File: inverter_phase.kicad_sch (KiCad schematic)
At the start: 34 parts, among them Q501 BSC072N08NS5, Q502 BSC072N08NS5, U501 IR2171S, U502 INA180B2

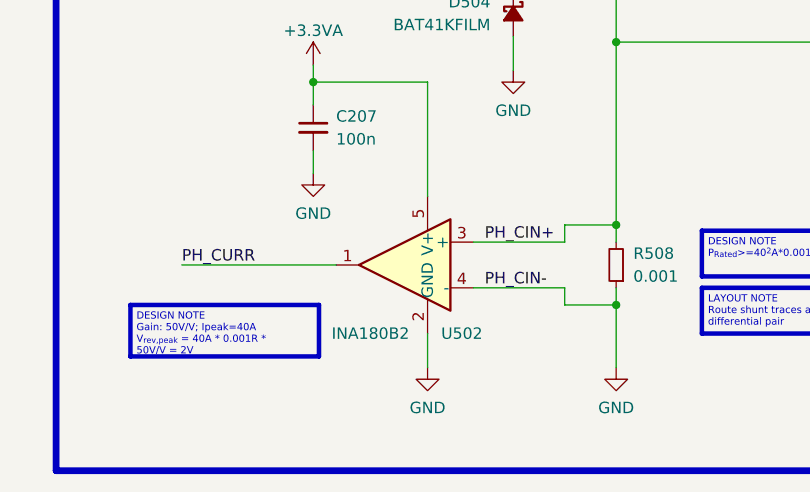
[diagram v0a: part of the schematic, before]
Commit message: feat: component placement, again
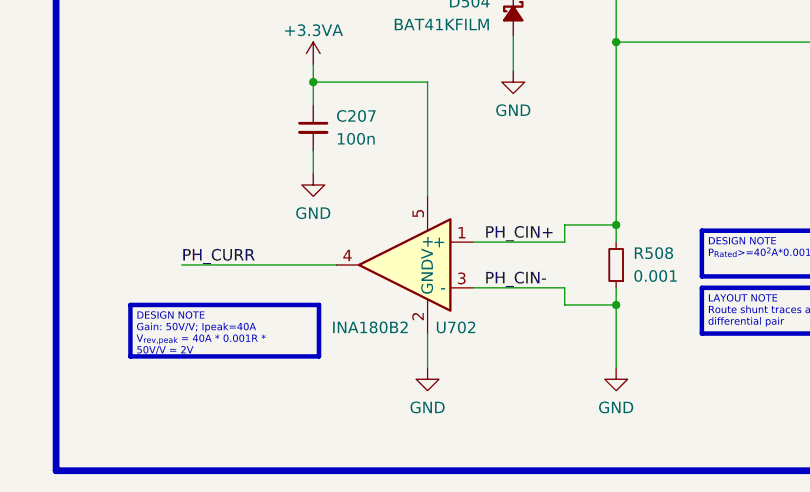
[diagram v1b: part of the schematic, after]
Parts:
- removed U502: INA180B2, Package_TO_SOT_SMD:SOT-23-5, symbol Amplifier_Current:INA180A2
- added U702: INA180B2, Package_TO_SOT_SMD:SOT-23-5, symbol Amplifier_Current:INA180B2
- C207: footprint Capacitor_SMD:C_0402_1005Metric_Pad0.74x0.62mm_HandSolder -> Capacitor_SMD:C_0805_2012Metric_Pad1.18x1.45mm_HandSolder
- C224: footprint Capacitor_SMD:C_0603_1608Metric_Pad1.08x0.95mm_HandSolder -> Capacitor_SMD:C_0805_2012Metric_Pad1.18x1.45mm_HandSolder
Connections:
- net +3.3VA: now also U702.5 (V+)
- net GND: now also U702.2 (GND), U702.3 (-)
- net PH_CIN+: now also U702.1 (+)
- net PH_CURR: now also U702.4
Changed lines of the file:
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@@
       (effects (font (size 1.27 1.27)) (justify left))
     )
-    (property "Footprint" "Capacitor_SMD:C_0402_1005Metric_Pad0.74x0.62mm_HandSolder" (at 257.175 86.995 0)
+    (property "Footprint" "Capacitor_SMD:C_0805_2012Metric_Pad1.18x1.45mm_HandSolder" (at 257.175 86.995 0)
       (effects (font (size 1.27 1.27)) hide)
     )
@@
       (effects (font (size 1.27 1.27)) (justify left))
     )
-    (property "Footprint" "Capacitor_SMD:C_0603_1608Metric_Pad1.08x0.95mm_HandSolder" (at 88.9 64.77 0)
+    (property "Footprint" "Capacitor_SMD:C_0805_2012Metric_Pad1.18x1.45mm_HandSolder" (at 88.9 64.77 0)
       (effects (font (size 1.27 1.27)) hide)
     )
@@
     )
   )
-  (symbol (lib_id "Device:C_Small") (at 102.235 64.77 180) (unit 1)
-    (in_bom yes) (on_board yes) (dnp no)
-    (property "Reference" "C502" (at 104.775 63.5 0)
-      (effects (font (size 1.27 1.27)) (justify right))
-    )
-    (property "Value" "100n 50V" (at 104.775 65.405 0)
-      (effects (font (size 1.27 1.27)) (justify right))
-    )
-    (property "Footprint" "Capacitor_SMD:C_0402_1005Metric_Pad0.74x0.62mm_HandSolder" (at 102.235 64.77 0)
-      (effects (font (size 1.27 1.27)) hide)
-    )
-    (property "Datasheet" "~" (at 102.235 64.77 0)
-      (effects (font (size 1.27 1.27)) hide)
-    )
-    (pin "1")
-    (pin "2")
-    (instances
-      (project "ESC_R1"
-        (path "/9dea2e18-5867-4ed4-a12d-7ee109225de0/a82201a8-9dca-4a1d-828e-2de3fb3c1adb"
-          (reference "C502") (unit 1)
-        )
-        (path "/9dea2e18-5867-4ed4-a12d-7ee109225de0/fe2fcbfe-ce2b-4fee-9243-f26c3dcbcd78"
-          (reference "C604") (unit 1)
-        )
-        (path "/9dea2e18-5867-4ed4-a12d-7ee109225de0/4eb0e494-3187-44db-9d3d-24d2fbf5dea7"
-          (reference "C704") (unit 1)
-        )
-      )
-    )
-  )
-  (symbol (lib_id "Device:C_Small") (at 107.95 139.065 180) (unit 1)
-    (in_bom yes) (on_board yes) (dnp no)
-    (property "Reference" "C509" (at 110.49 138.43 0)
-      (effects (font (size 1.27 1.27)) (justify right))
-    )
-    (property "Value" "10n" (at 110.49 140.335 0)
-      (effects (font (size 1.27 1.27)) (justify right))
-    )
-    (property "Footprint" "Capacitor_SMD:C_0603_1608Metric_Pad1.08x0.95mm_HandSolder" (at 107.95 139.065 0)
-      (effects (font (size 1.27 1.27)) hide)
-    )
-    (property "Datasheet" "~" (at 107.95 139.065 0)
-      (effects (font (size 1.27 1.27)) hide)
-    )
-    (pin "1")
-    (pin "2")
-    (instances
-      (project "ESC_R1"
-        (path "/9dea2e18-5867-4ed4-a12d-7ee109225de0/a82201a8-9dca-4a1d-828e-2de3fb3c1adb"
-          (reference "C509") (unit 1)
-        )
-        (path "/9dea2e18-5867-4ed4-a12d-7ee109225de0/fe2fcbfe-ce2b-4fee-9243-f26c3dcbcd78"
-          (reference "C609") (unit 1)
-        )
-        (path "/9dea2e18-5867-4ed4-a12d-7ee109225de0/4eb0e494-3187-44db-9d3d-24d2fbf5dea7"
-          (reference "C709") (unit 1)
-        )
-      )
-    )
-  )
-  (symbol (lib_id "Amplifier_Current:INA180A2") (at 207.645 138.43 0) (mirror y) (unit 1)
-    (in_bom yes) (on_board yes) (dnp no)
-    (property "Reference" "U502" (at 213.995 146.05 0)
-      (effects (font (size 1.27 1.27)))
-    )
-    (property "Value" "INA180B2" (at 203.835 146.05 0)
-      (effects (font (size 1.27 1.27)))
-    )
-    (property "Footprint" "Package_TO_SOT_SMD:SOT-23-5" (at 206.375 137.16 0)
-      (effects (font (size 1.27 1.27)) hide)
-    )
-    (property "Datasheet" "http://www.ti.com/lit/ds/symlink/ina180.pdf" (at 203.835 134.62 0)
-      (effects (font (size 1.27 1.27)) hide)
-    )
-    (property "Link" "https://www.digikey.de/en/products/detail/texas-instruments/INA180B2IDBVR/8105877" (at 207.645 138.43 0)
+  (symbol (lib_id "Amplifier_Current:INA180B2") (at 210.185 138.43 0) (mirror y) (unit 1)
+    (in_bom yes) (on_board yes) (dnp no)
+    (property "Reference" "U702" (at 213.36 145.415 0)
+      (effects (font (size 1.27 1.27)))
+    )
+    (property "Value" "INA180B2" (at 203.835 145.415 0)
+      (effects (font (size 1.27 1.27)))
+    )
+    (property "Footprint" "Package_TO_SOT_SMD:SOT-23-5" (at 210.185 138.43 0)
+      (effects (font (size 1.27 1.27)) hide)
+    )
+    (property "Datasheet" "" (at 210.185 138.43 0)
+      (effects (font (size 1.27 1.27)) hide)
+    )
+    (property "Link" "https://www.digikey.de/en/products/detail/texas-instruments/INA180B2IDBVR/8105877" (at 210.185 138.43 0)
       (effects (font (size 1.27 1.27)) hide)
     )
@@
     (instances
       (project "ESC_R1"
+        (path "/9dea2e18-5867-4ed4-a12d-7ee109225de0/4eb0e494-3187-44db-9d3d-24d2fbf5dea7"
+          (reference "U702") (unit 1)
+        )
         (path "/9dea2e18-5867-4ed4-a12d-7ee109225de0/a82201a8-9dca-4a1d-828e-2de3fb3c1adb"
           (reference "U502") (unit 1)
@@
           (reference "U602") (unit 1)
         )
-        (path "/9dea2e18-5867-4ed4-a12d-7ee109225de0/4eb0e494-3187-44db-9d3d-24d2fbf5dea7"
-          (reference "U702") (unit 1)
-        )
-      )
+      )
+    )
+  )
+  (symbol (lib_id "Device:C_Small") (at 102.235 64.77 180) (unit 1)
+    (in_bom yes) (on_board yes) (dnp no)
+    (property "Reference" "C502" (at 104.775 63.5 0)
+      (effects (font (size 1.27 1.27)) (justify right))
+    )
+    (property "Value" "100n 50V" (at 104.775 65.405 0)
+      (effects (font (size 1.27 1.27)) (justify right))
+    )
+    (property "Footprint" "Capacitor_SMD:C_0402_1005Metric_Pad0.74x0.62mm_HandSolder" (at 102.235 64.77 0)
+      (effects (font (size 1.27 1.27)) hide)
+    )
+    (property "Datasheet" "~" (at 102.235 64.77 0)
+      (effects (font (size 1.27 1.27)) hide)
+    )
+    (pin "1")
+    (pin "2")
+    (instances
+      (project "ESC_R1"
+        (path "/9dea2e18-5867-4ed4-a12d-7ee109225de0/a82201a8-9dca-4a1d-828e-2de3fb3c1adb"
+          (reference "C502") (unit 1)
+        )
+        (path "/9dea2e18-5867-4ed4-a12d-7ee109225de0/fe2fcbfe-ce2b-4fee-9243-f26c3dcbcd78"
+          (reference "C604") (unit 1)
+        )
+        (path "/9dea2e18-5867-4ed4-a12d-7ee109225de0/4eb0e494-3187-44db-9d3d-24d2fbf5dea7"
+          (reference "C704") (unit 1)
+        )
+      )
+    )
+  )
+  (symbol (lib_id "Device:C_Small") (at 107.95 139.065 180) (unit 1)
+    (in_bom yes) (on_board yes) (dnp no)
+    (property "Reference" "C509" (at 110.49 138.43 0)
+      (effects (font (size 1.27 1.27)) (justify right))
+    )
+    (property "Value" "10n" (at 110.49 140.335 0)
+      (effects (font (size 1.27 1.27)) (justify right))
+    )
+    (property "Footprint" "Capacitor_SMD:C_0603_1608Metric_Pad1.08x0.95mm_HandSolder" (at 107.95 139.065 0)
+      (effects (font (size 1.27 1.27)) hide)
+    )
+    (property "Datasheet" "~" (at 107.95 139.065 0)
+      (effects (font (size 1.27 1.27)) hide)
+    )
+    (pin "1")
+    (pin "2")
+    (instances
+      (project "ESC_R1"
+        (path "/9dea2e18-5867-4ed4-a12d-7ee109225de0/a82201a8-9dca-4a1d-828e-2de3fb3c1adb"
+          (reference "C509") (unit 1)
+        )
+        (path "/9dea2e18-5867-4ed4-a12d-7ee109225de0/fe2fcbfe-ce2b-4fee-9243-f26c3dcbcd78"
+          (reference "C609") (unit 1)
+        )
+        (path "/9dea2e18-5867-4ed4-a12d-7ee109225de0/4eb0e494-3187-44db-9d3d-24d2fbf5dea7"
+          (reference "C709") (unit 1)
+        )
+      )
